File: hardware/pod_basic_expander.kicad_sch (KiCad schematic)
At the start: 7 parts, among them J1 POD, SW1 SW_MEC_5E, SW2 SW_MEC_5E, SW3 SW_MEC_5E, SW4 SW_MEC_5E

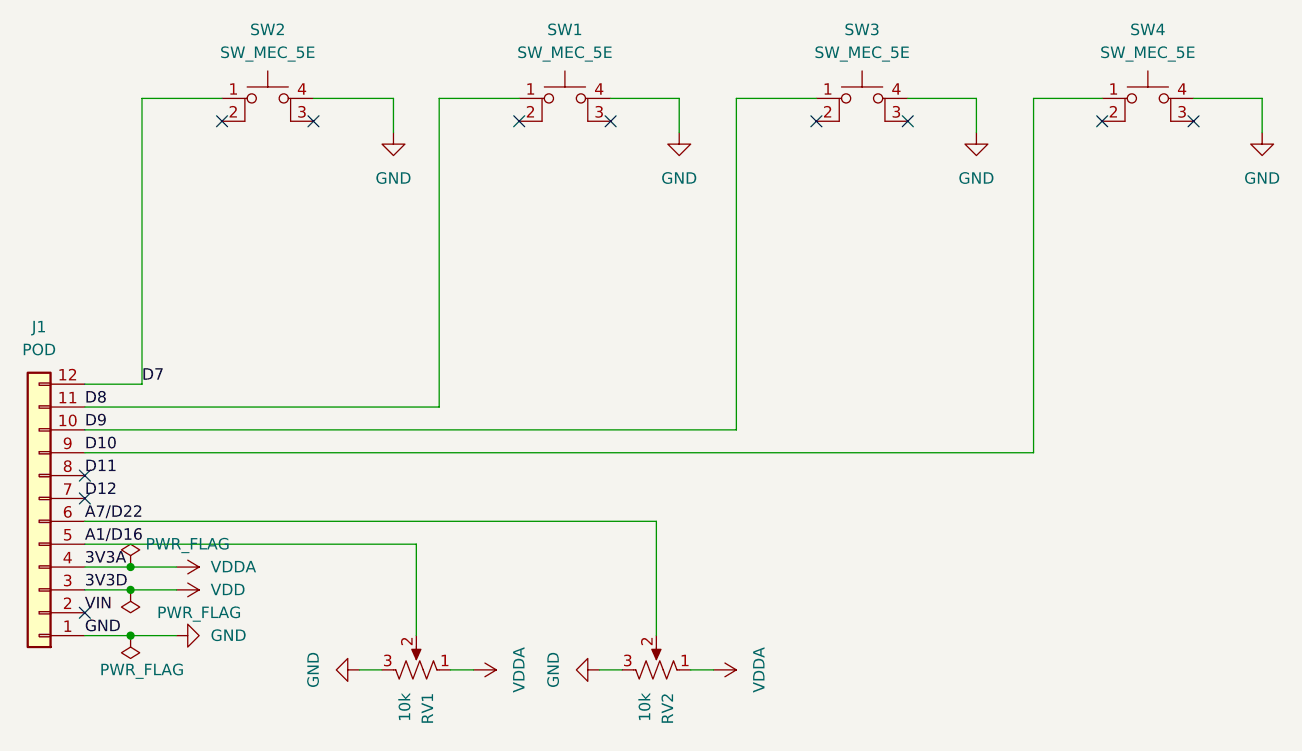
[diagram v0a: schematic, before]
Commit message: PCB changes
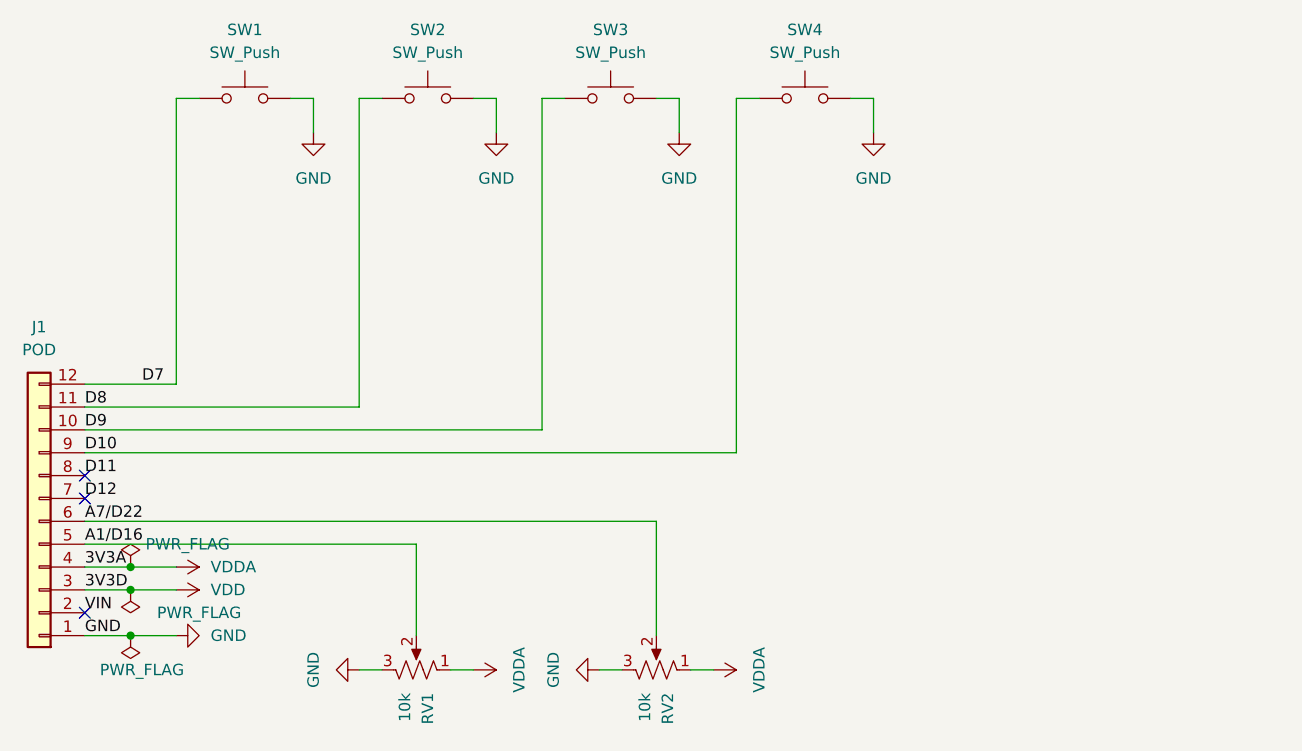
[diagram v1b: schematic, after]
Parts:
- removed SW1, SW2, SW3, SW4: SW_MEC_5E, Button_Switch_THT:SW_PUSH_6mm, symbol Switch:SW_MEC_5E
- added SW1, SW2, SW3, SW4: SW_Push, Button_Switch_THT:SW_PUSH_6mm, symbol Switch:SW_Push
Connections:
- net D10: now also SW4.1
- net D7: now also SW1.1
- net D8: now also SW2.1
- net D9: now also SW3.1
- net GND: now also SW1.2, SW2.2, SW3.2, SW4.2
- no-connect marks 11 -> 3
